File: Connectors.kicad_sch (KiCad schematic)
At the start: 6 parts, among them J1 Motor, J2 DJI_VTX, J3 GPS, J4 CRSF_Receiver, J5 Analog_Camera, J6 Analog_VTX

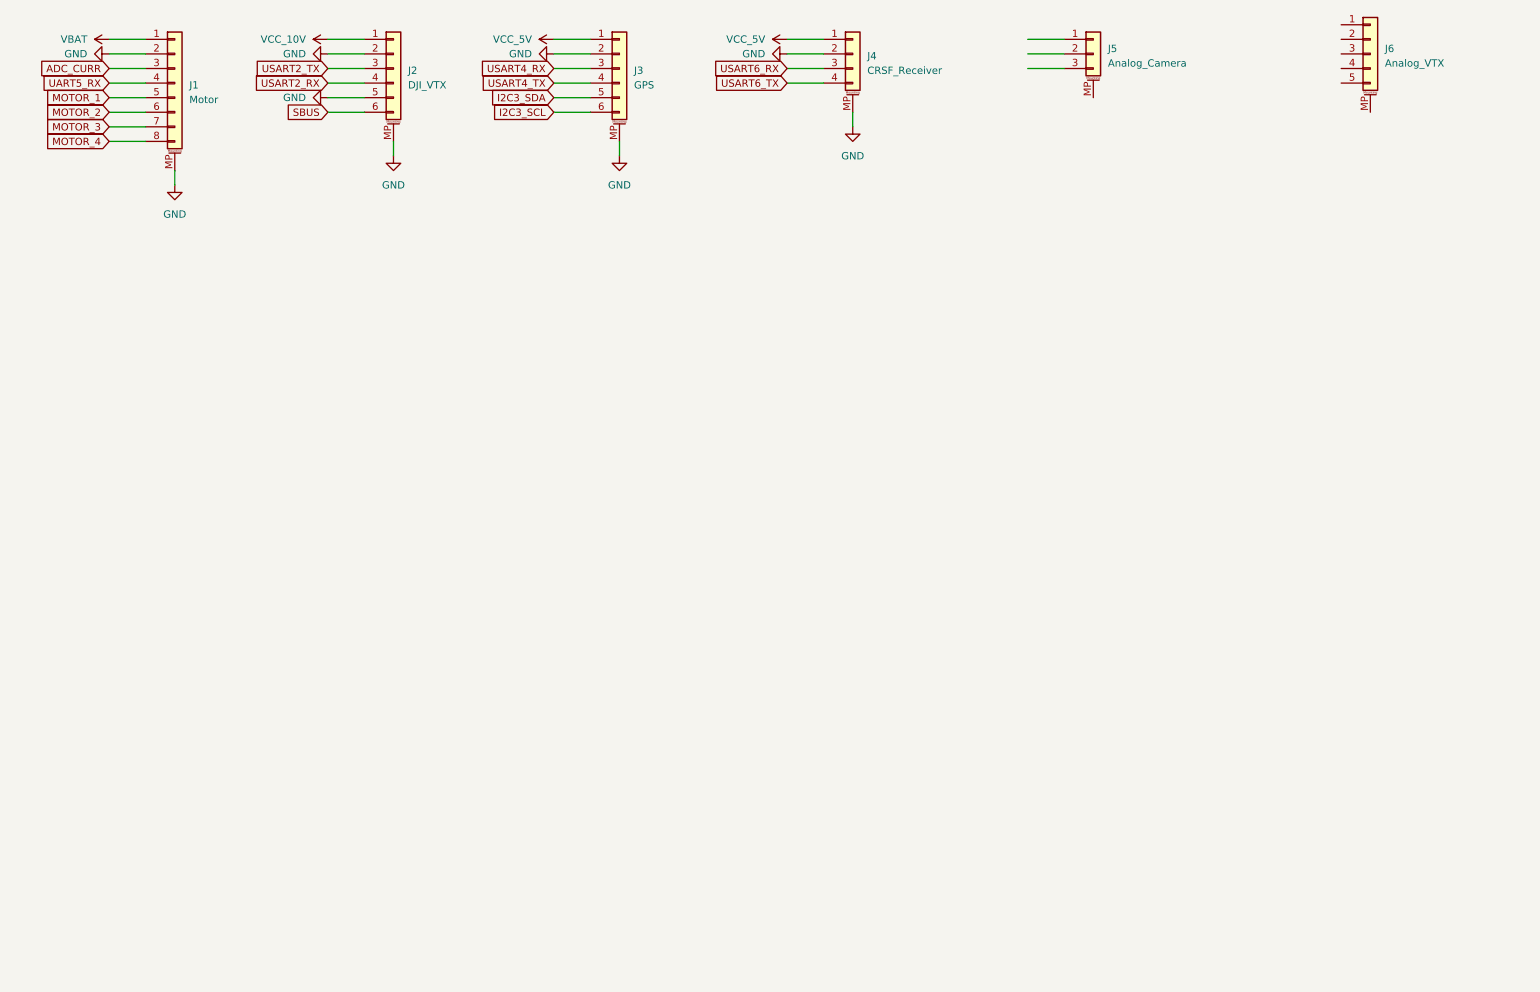
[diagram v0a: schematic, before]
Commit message: Finished SCH
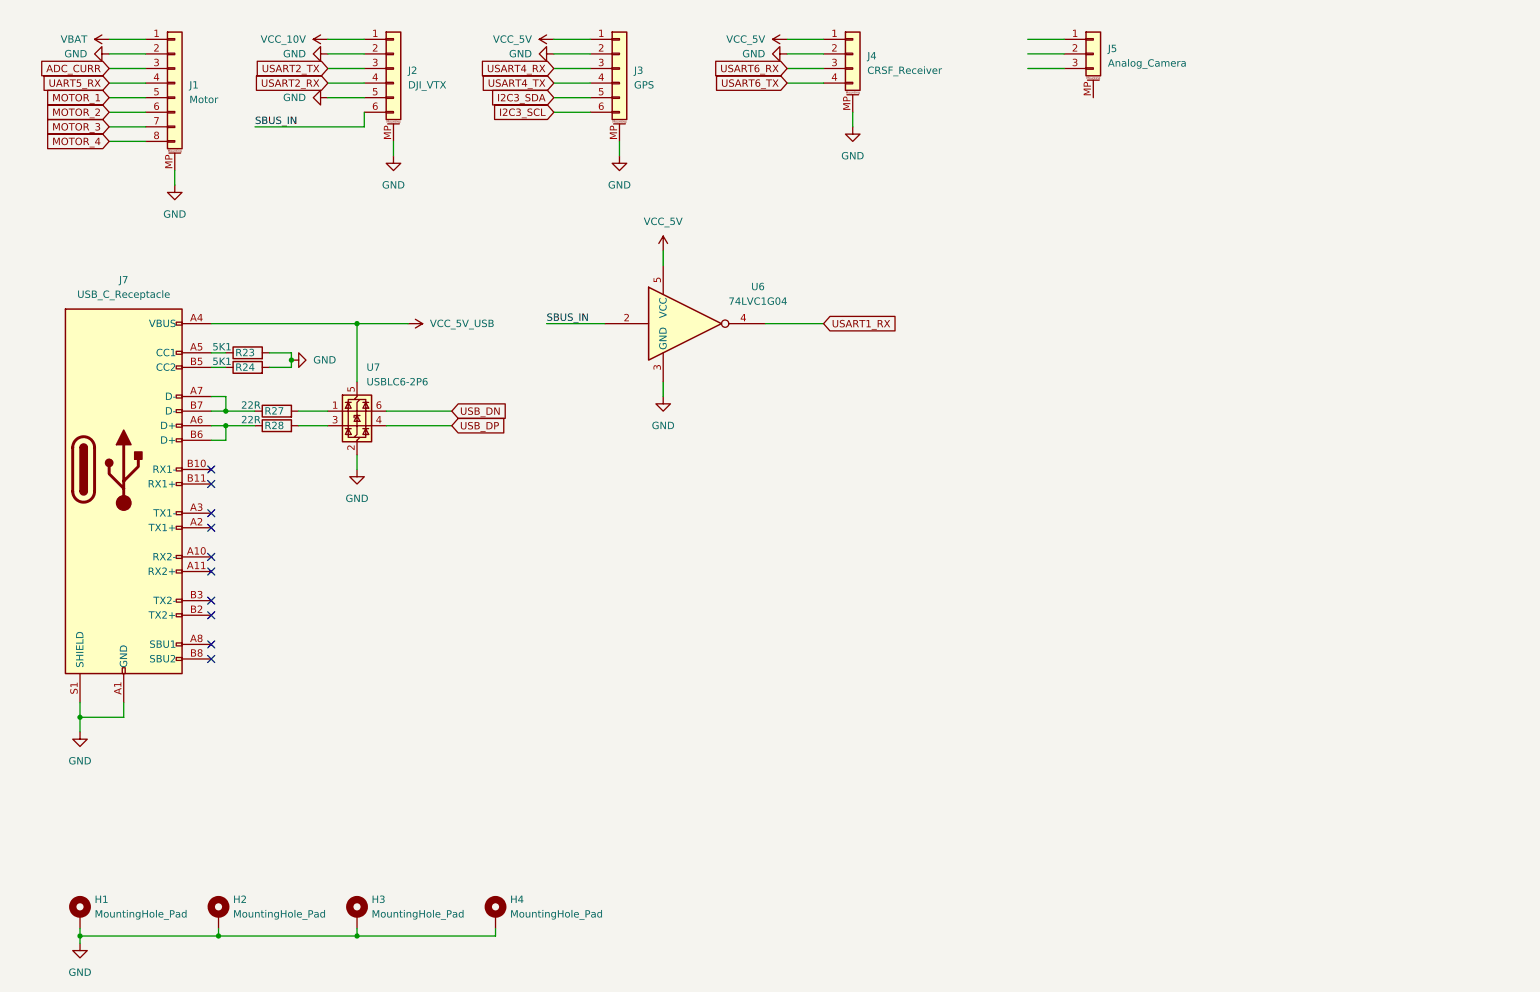
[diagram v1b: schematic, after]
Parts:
- removed J6: Analog_VTX, Connector_JST:JST_SH_SM05B-SRSS-TB_1x05-1MP_P1.00mm_Horizontal, symbol Library:Conn_01x05_MountingPin
- added H1, H2, H3, H4: MountingHole_Pad, MountingHole:MountingHole_3.2mm_M3_DIN965_Pad, symbol Mechanical:MountingHole_Pad
- added J7: USB_C_Receptacle, SamacSys_Parts:USB-C_halfboard, symbol Connector:USB_C_Receptacle
- added R23, R24: 5K1, Resistor_SMD:R_0402_1005Metric, symbol Library:R
- added R27, R28: 22R, Resistor_SMD:R_0402_1005Metric, symbol Library:R
- added U6: 74LVC1G04, Package_TO_SOT_SMD:SOT-23-5, symbol 74xGxx:74LVC1G04
- added U7: USBLC6-2P6, Package_TO_SOT_SMD:SOT-666, symbol Power_Protection:USBLC6-2P6
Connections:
- net GND: now also H1.1, H2.1, H3.1, H4.1, J7.A1 (GND), J7.A12 (GND), J7.B1 (GND), J7.B12 (GND), J7.S1 (SHIELD), R23.2, R24.2, U6.3 (GND), U7.2 (GND)
- net VCC_5V: now also U6.5 (VCC)
- net SBUS renamed SBUS_IN
- net SBUS_IN: now also U6.2
- new net: J7.A7 (D-), J7.B7 (D-), R27.1
- new net: R27.2, U7.1 (I/O1)
- new net: J7.A5 (CC1), R23.1
- new net: J7.B5 (CC2), R24.1
- new net: J7.A6 (D+), J7.B6 (D+), R28.1
- new net: R28.2, U7.3 (I/O2)
- new net USART1_RX: U6.4
- new net USB_DN: U7.6 (I/O1)
- new net USB_DP: U7.4 (I/O2)
- new net VCC_5V_USB: J7.A4 (VBUS), J7.A9 (VBUS), J7.B4 (VBUS), J7.B9 (VBUS), U7.5 (VBUS)
- no-connect marks 0 -> 10

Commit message: Updated PCB Layout
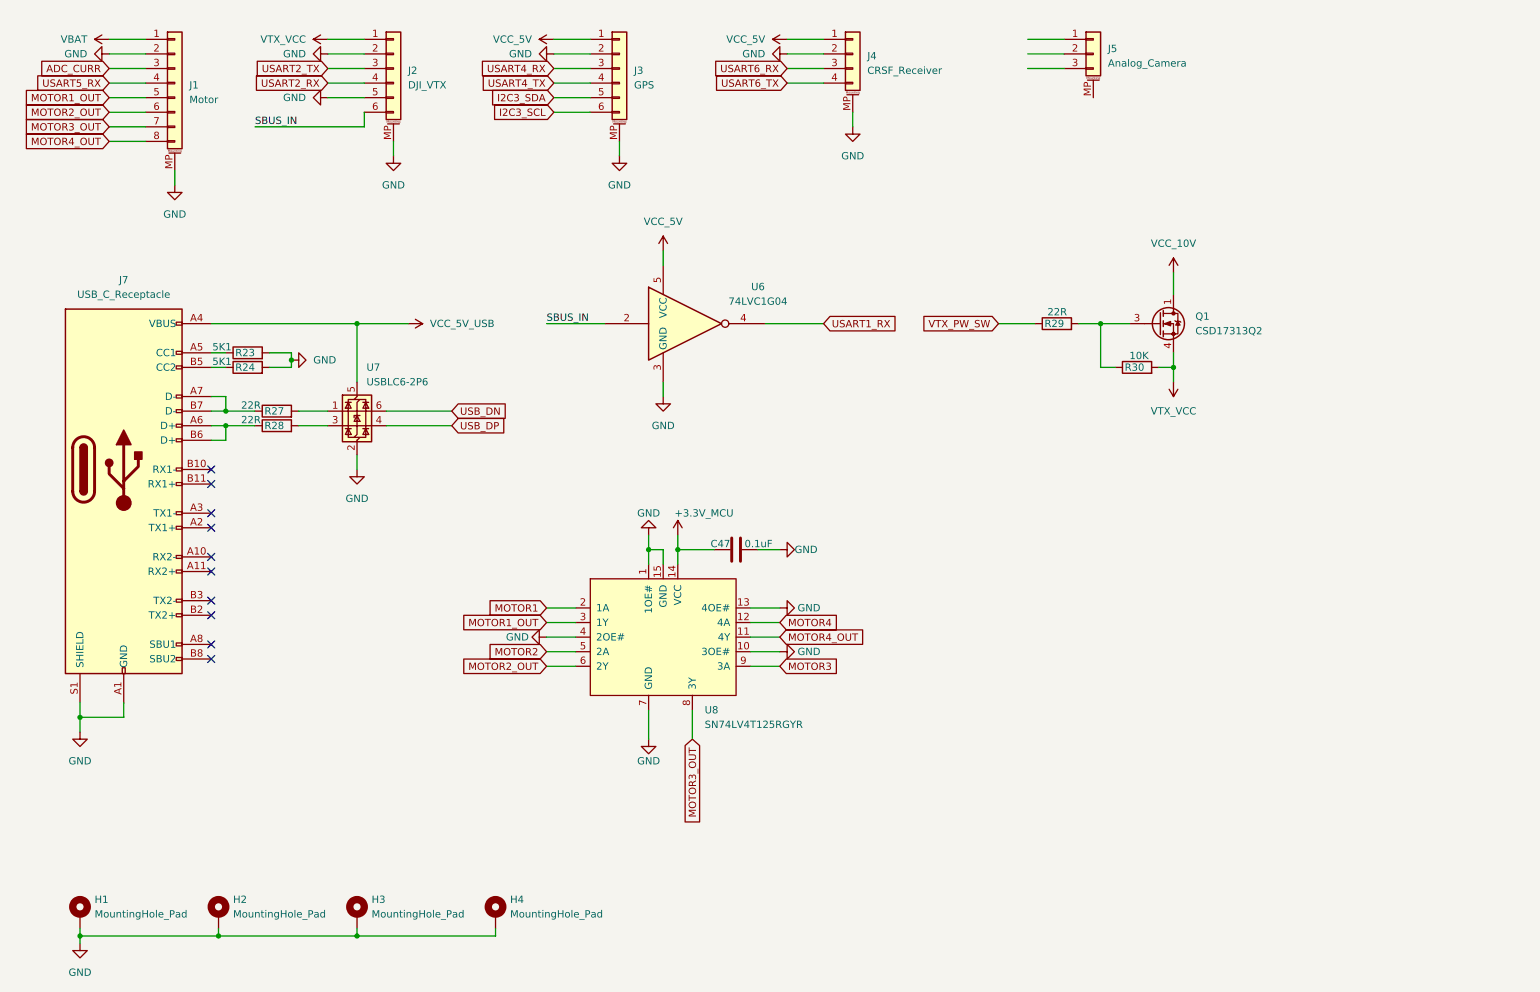
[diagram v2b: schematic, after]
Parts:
- added C47: 0.1uF, Capacitor_SMD:C_0402_1005Metric, symbol Library:C
- added Q1: CSD17313Q2, Package_SON:Texas_DQK, symbol Transistor_FET:CSD17313Q2
- added R29: 22R, Resistor_SMD:R_0402_1005Metric, symbol Library:R
- added R30: 10K, Resistor_SMD:R_0402_1005Metric, symbol Library:R
- added U8: SN74LV4T125RGYR, Library:VQFN-14_L3.5-W3.5-P0.50-BL-EP, symbol Library:SN74LV4T125RGYR
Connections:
- net GND: now also C47.2, U8.1 (1OE#), U8.10 (3OE#), U8.13 (4OE#), U8.15 (GND), U8.4 (2OE#), U8.7 (GND)
- net VCC_10V: now also Q1.1 (D), Q1.2 (D), Q1.5 (D), Q1.6 (D), Q1.8 (D); no longer J2.1 (Pin_1)
- net MOTOR_1 renamed MOTOR1_OUT
- net MOTOR1_OUT: now also U8.3 (1Y)
- net MOTOR_2 renamed MOTOR2_OUT
- net MOTOR2_OUT: now also U8.6 (2Y)
- net MOTOR_3 renamed MOTOR3_OUT
- net MOTOR3_OUT: now also U8.8 (3Y)
- net MOTOR_4 renamed MOTOR4_OUT
- net MOTOR4_OUT: now also U8.11 (4Y)
- net UART5_RX renamed USART5_RX
- new net: Q1.3 (G), R29.2, R30.1
- new net +3.3V_MCU: C47.1, U8.14 (VCC)
- new net MOTOR1: U8.2 (1A)
- new net MOTOR2: U8.5 (2A)
- new net MOTOR3: U8.9 (3A)
- new net MOTOR4: U8.12 (4A)
- new net VTX_PW_SW: R29.1
- new net VTX_VCC: J2.1 (Pin_1), Q1.4 (S), Q1.7 (S), R30.2

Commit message: Update PCB Layout
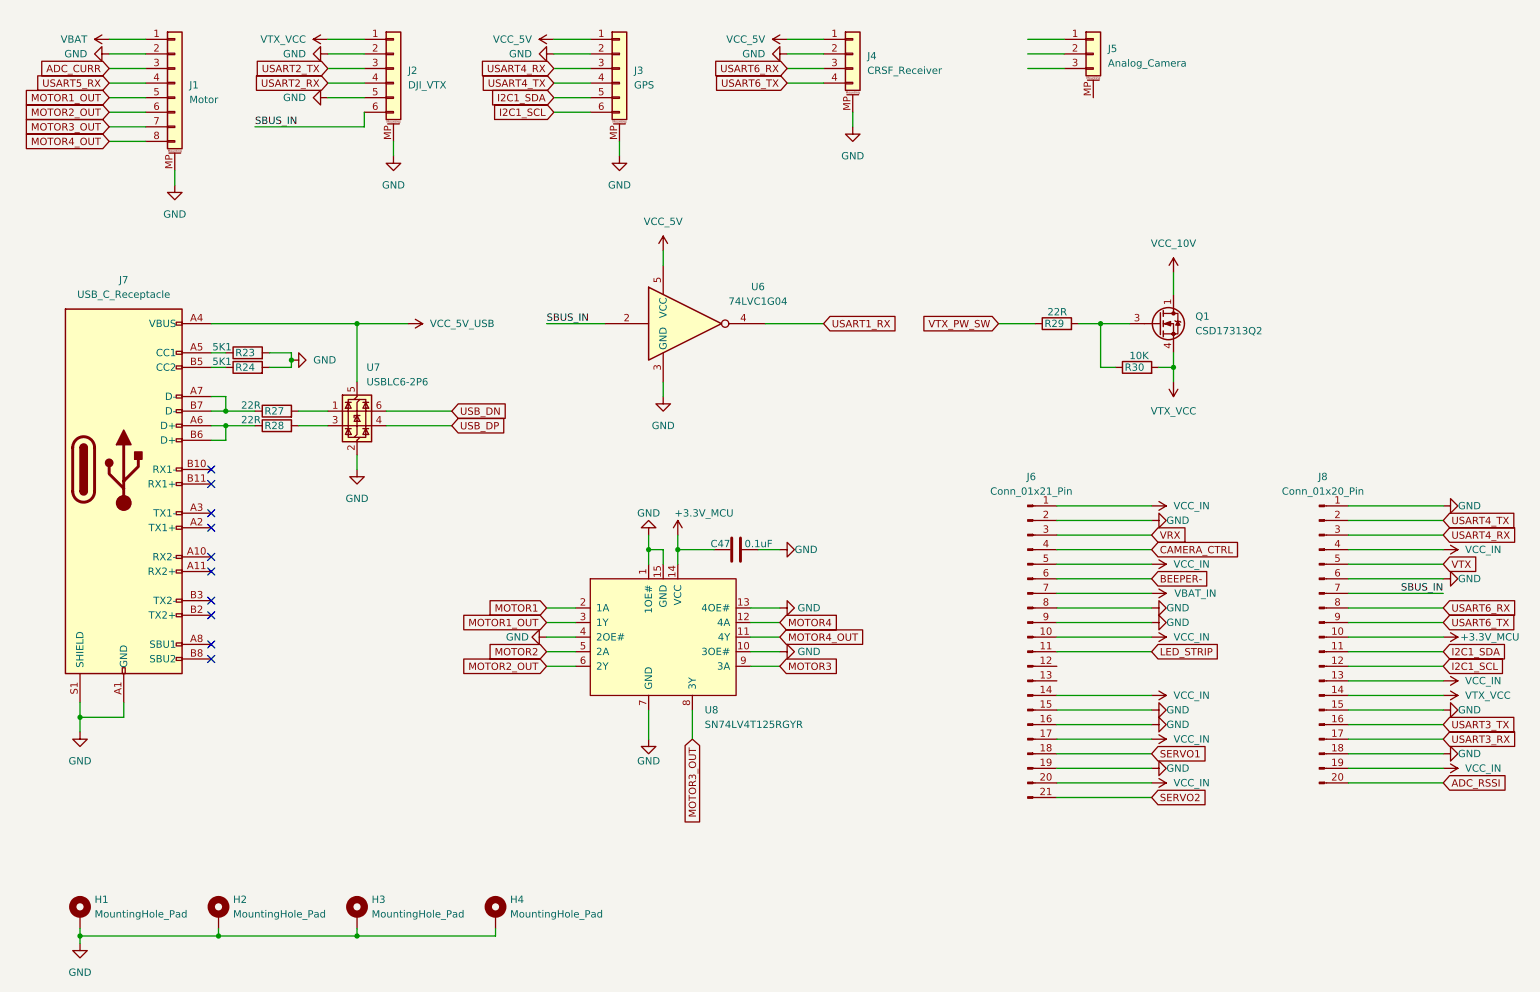
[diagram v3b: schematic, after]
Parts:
- added J6: Conn_01x21_Pin, Library:Betaflight_Pad_F, symbol Connector:Conn_01x21_Pin
- added J8: Conn_01x20_Pin, Library:Betaflight_Pad_B, symbol Connector:Conn_01x20_Pin
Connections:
- net +3.3V_MCU: now also J8.10 (Pin_10)
- net GND: now also J6.15 (Pin_15), J6.16 (Pin_16), J6.19 (Pin_19), J6.2 (Pin_2), J6.8 (Pin_8), J6.9 (Pin_9), J8.1 (Pin_1), J8.15 (Pin_15), J8.18 (Pin_18), J8.6 (Pin_6)
- net SBUS_IN: now also J8.7 (Pin_7)
- net USART4_RX: now also J8.3 (Pin_3)
- net USART4_TX: now also J8.2 (Pin_2)
- net USART6_RX: now also J8.8 (Pin_8)
- net USART6_TX: now also J8.9 (Pin_9)
- net VTX_VCC: now also J8.14 (Pin_14)
- net I2C3_SCL renamed I2C1_SCL
- net I2C1_SCL: now also J8.12 (Pin_12)
- net I2C3_SDA renamed I2C1_SDA
- net I2C1_SDA: now also J8.11 (Pin_11)
- new net ADC_RSSI: J8.20 (Pin_20)
- new net BEEPER-: J6.6 (Pin_6)
- new net CAMERA_CTRL: J6.4 (Pin_4)
- new net LED_STRIP: J6.11 (Pin_11)
- new net SERVO1: J6.18 (Pin_18)
- new net SERVO2: J6.21 (Pin_21)
- new net USART3_RX: J8.17 (Pin_17)
- new net USART3_TX: J8.16 (Pin_16)
- new net VBAT_IN: J6.7 (Pin_7)
- new net VCC_IN: J6.1 (Pin_1), J6.10 (Pin_10), J6.14 (Pin_14), J6.17 (Pin_17), J6.20 (Pin_20), J6.5 (Pin_5), J8.13 (Pin_13), J8.19 (Pin_19), J8.4 (Pin_4)
- new net VRX: J6.3 (Pin_3)
- new net VTX: J8.5 (Pin_5)

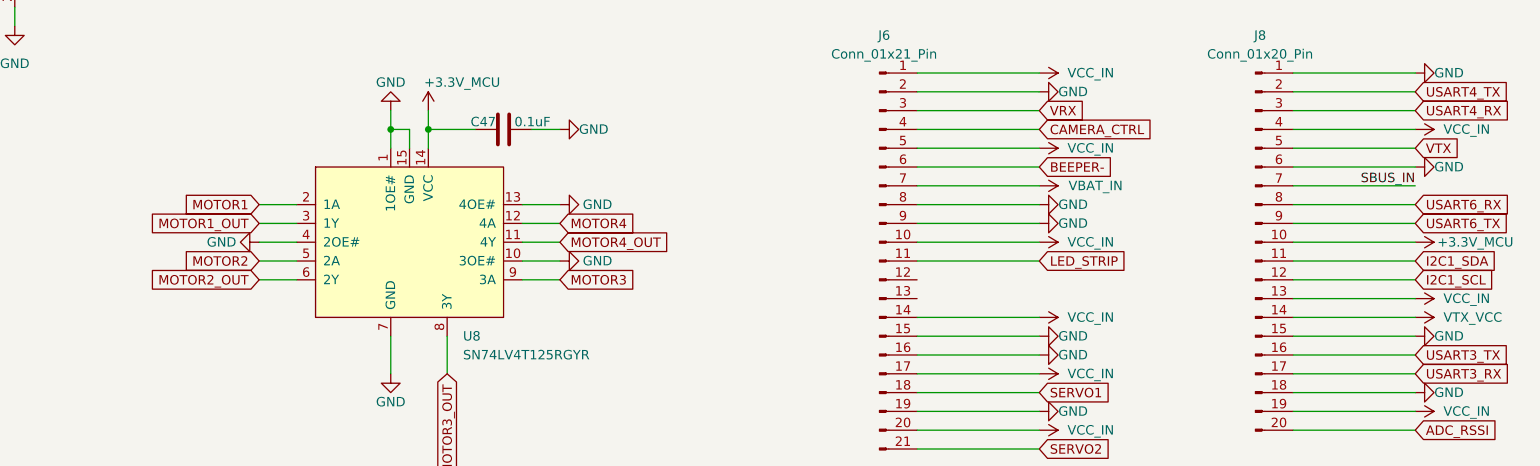
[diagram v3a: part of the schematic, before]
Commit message: Updated PCB Layout
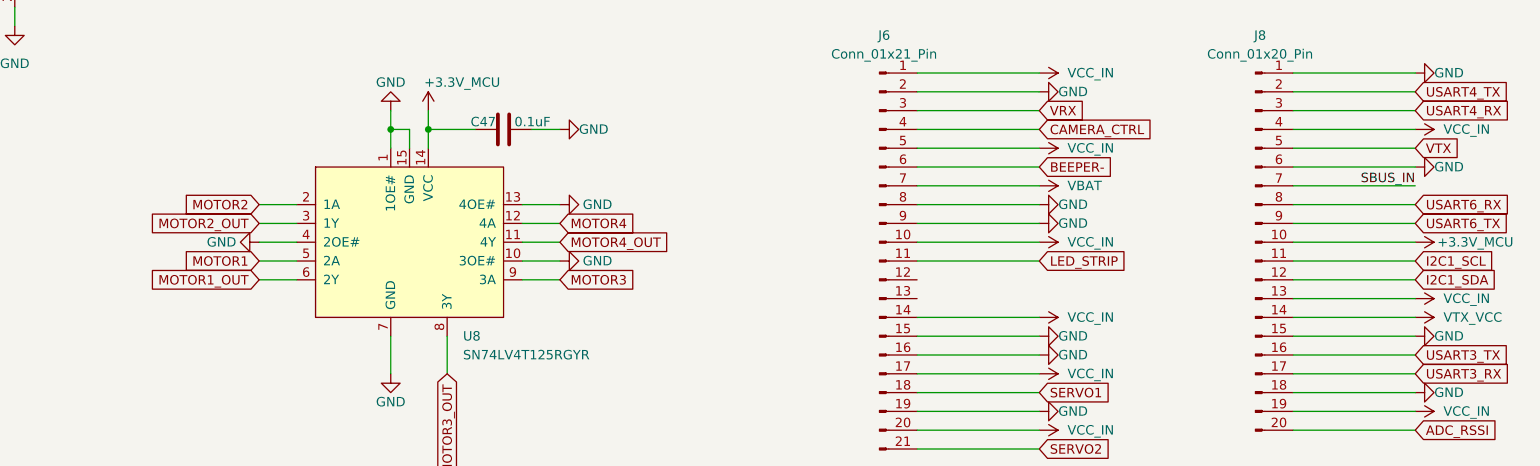
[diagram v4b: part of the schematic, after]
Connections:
- net VBAT_IN is gone; now on net VBAT: J6.7 (Pin_7)
- net I2C1_SCL: now also J8.11 (Pin_11); no longer J8.12 (Pin_12)
- net I2C1_SDA: now also J8.12 (Pin_12); no longer J8.11 (Pin_11)
- net MOTOR1: now also U8.5 (2A); no longer U8.2 (1A)
- net MOTOR1_OUT: now also U8.6 (2Y); no longer U8.3 (1Y)
- net MOTOR2: now also U8.2 (1A); no longer U8.5 (2A)
- net MOTOR2_OUT: now also U8.3 (1Y); no longer U8.6 (2Y)
